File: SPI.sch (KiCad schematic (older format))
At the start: 7 parts

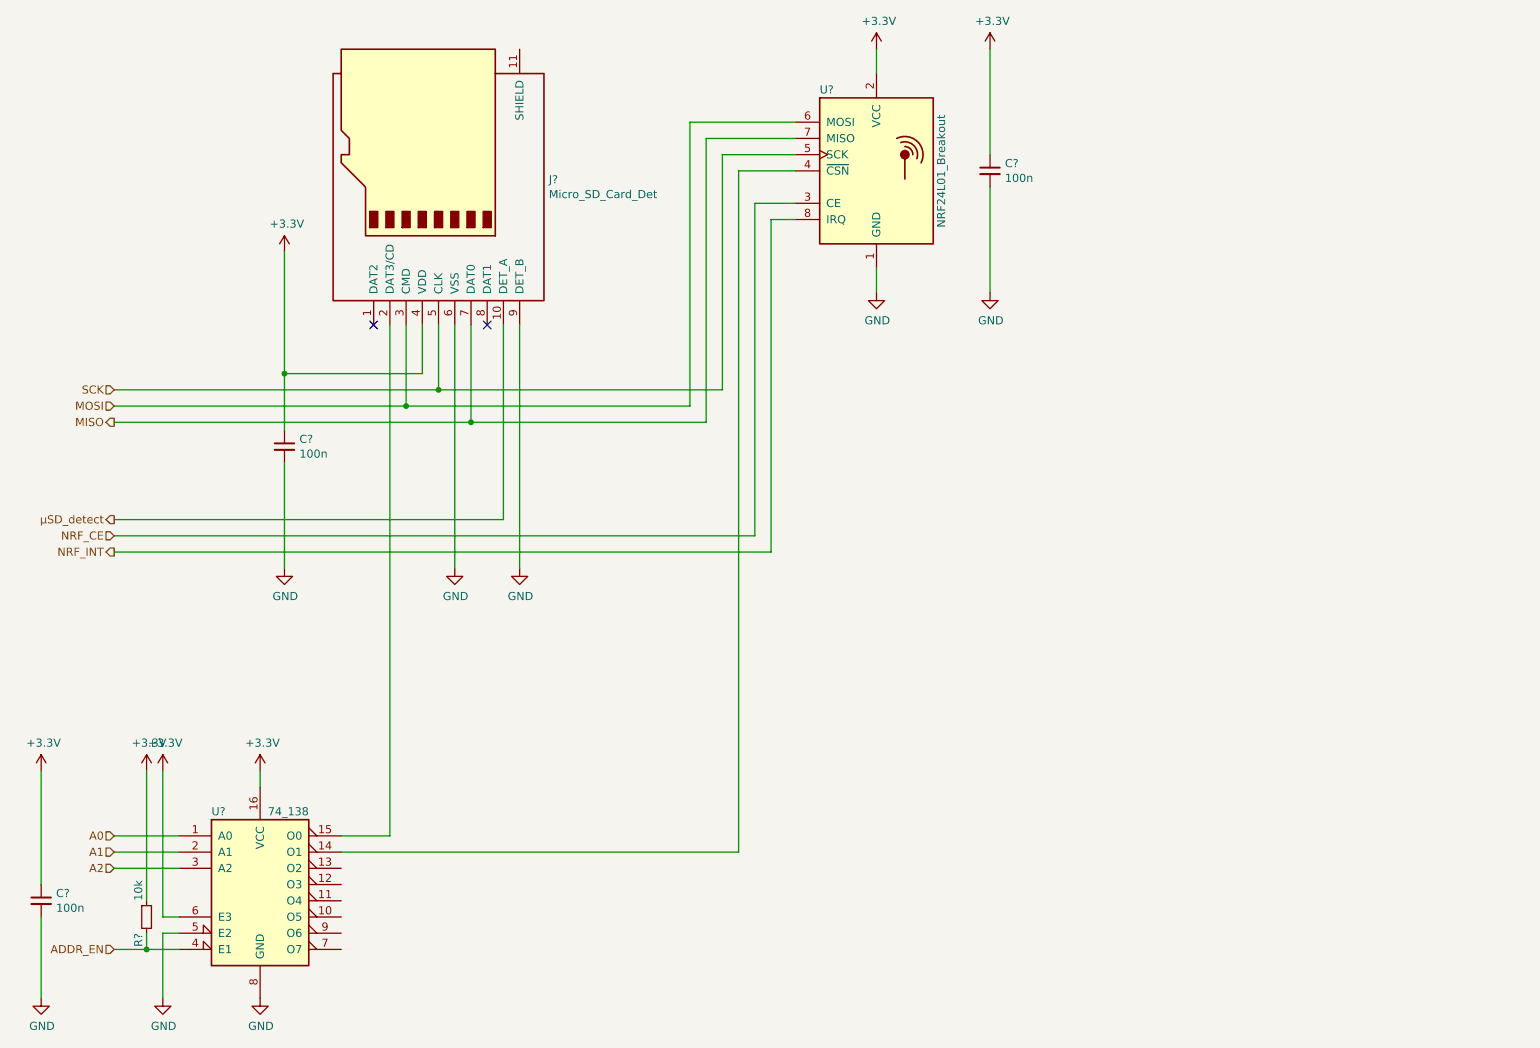
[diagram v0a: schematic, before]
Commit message: Erste fertige Version
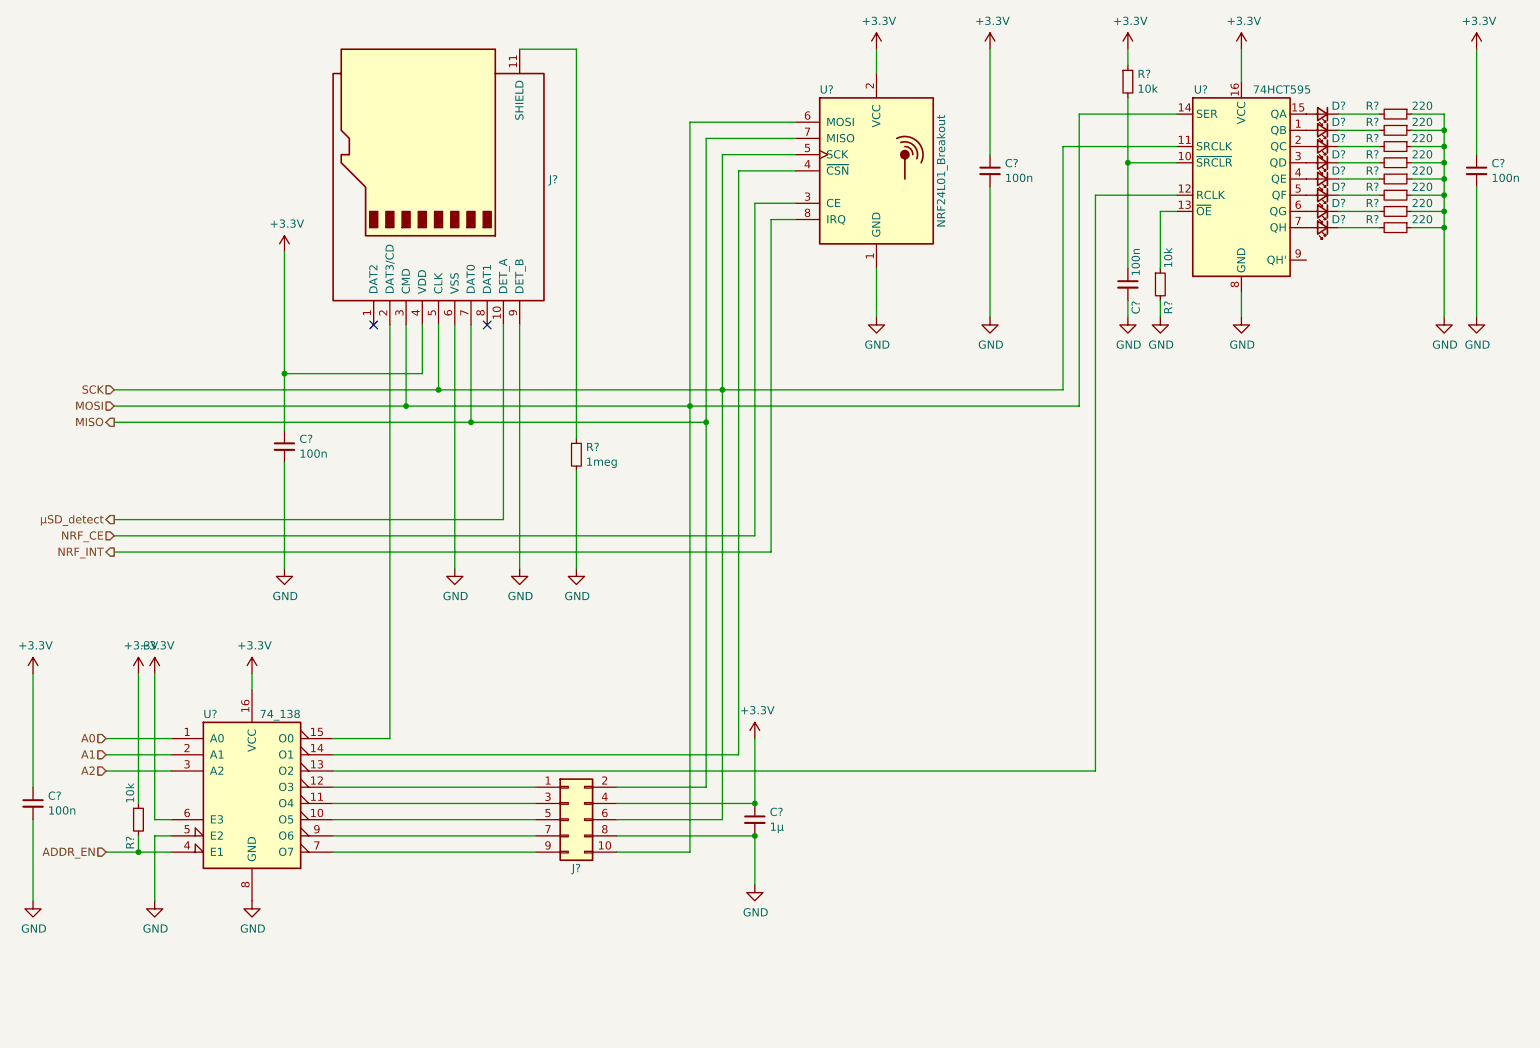
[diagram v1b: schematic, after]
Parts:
- added C? (x2): 100n, symbol Device:C_Small
- added C?: 1µ, symbol Device:C_Small
- added D? (x8): LED_Small, symbol Device:LED_Small
- added J?: Conn_02x05_Odd_Even, symbol Connector_Generic:Conn_02x05_Odd_Even
- added R?: 1meg, symbol Device:R_Small
- added R? (x2): 10k, symbol Device:R_Small
- added R? (x8): 220, symbol Device:R_Small
- added U?: 74HCT595, symbol 74xx:74HCT595
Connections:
- net +3V3: now also C?.1, C?.1, J?.4 (Pin_4), R?.1, U?.16 (VCC)
- net GND: now also C?.2, C?.2, C?.2, J?.8 (Pin_8), R?.1, R?.1, R?.1, R?.1, R?.1, R?.1, R?.1, R?.1, R?.2, R?.2, U?.8 (GND)
- net MISO: now also J?.2 (Pin_2)
- net MOSI: now also J?.10 (Pin_10), U?.14 (SER)
- net SCK: now also J?.6 (Pin_6), U?.11 (SRCLK)
- net at U?.10 (O5): now also J?.5 (Pin_5)
- net at U?.11 (O4): now also J?.3 (Pin_3)
- net at U?.12 (O3): now also J?.1 (Pin_1)
- net at U?.13 (O2): now also U?.12 (RCLK)
- net at U?.7 (O7): now also J?.9 (Pin_9)
- net at U?.9 (O6): now also J?.7 (Pin_7)
- net at J?.11 (SHIELD): now also R?.1
- new net: D?.2 (A), U?.1 (QB)
- new net: C?.1, R?.2, U?.10 (~SRCLR)
- new net: R?.1, U?.13 (~OE)
- new net: D?.2 (A), U?.15 (QA)
- new net: D?.2 (A), U?.2 (QC)
- new net: D?.2 (A), U?.3 (QD)
- new net: D?.2 (A), U?.4 (QE)
- new net: D?.2 (A), U?.5 (QF)
- new net: D?.2 (A), U?.6 (QG)
- new net: D?.2 (A), U?.7 (QH)
- new net: D?.1 (K), R?.2 (x8)
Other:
- moved on the sheet: C?, R?, U?
